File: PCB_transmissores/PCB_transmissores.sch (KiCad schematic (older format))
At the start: 17 parts, among them J2 Barrel_Jack_MountingPin

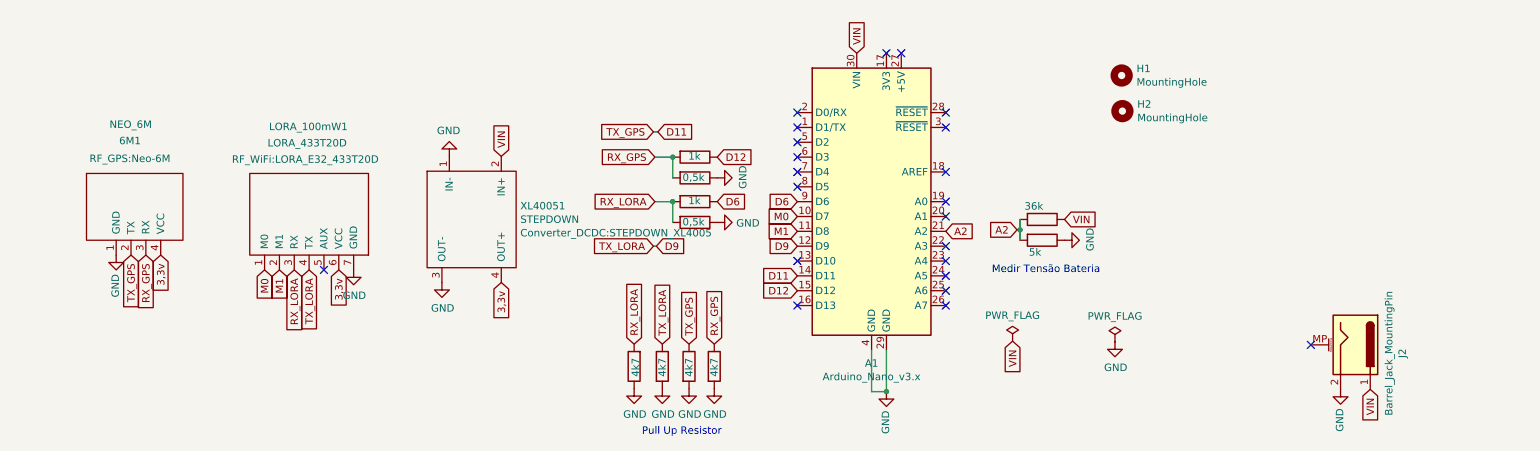
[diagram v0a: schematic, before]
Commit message: Atualização placa dos transmissores
Up
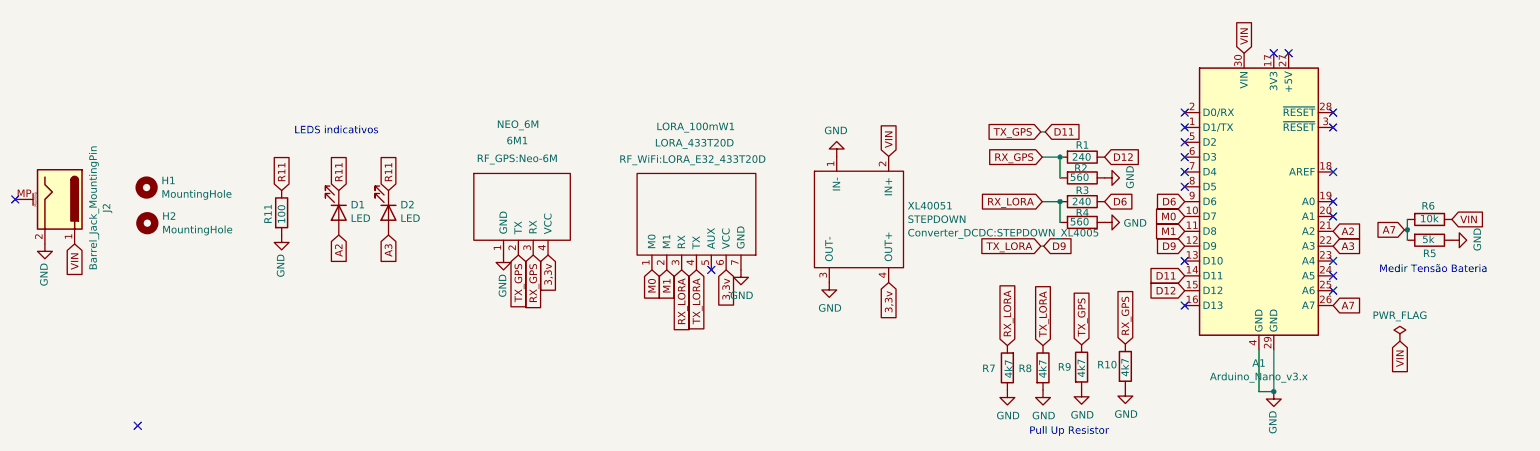
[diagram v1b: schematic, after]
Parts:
- added D1, D2: LED, LED_THT:LED_D5.0mm, symbol Device:LED
- added R11: 100, Resistor_THT:R_Axial_DIN0207_L6.3mm_D2.5mm_P7.62mm_Horizontal, symbol Device:R
- R1, R3: value 1k -> 240
- R2, R4: value 0,5k -> 560
- R6: value 36k -> 10k
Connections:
- net A2: now also D1.2 (A); no longer R5.2, R6.2
- net GND: now also R11.2
- net A3: now reaches A1.22 (A3)
- net A3: now also D2.2 (A)
- net A7: now reaches A1.26 (A7)
- net A7: now also R5.2, R6.2
- new net R11: D1.1 (K), D2.1 (K), R11.1
- no-connect marks 22 -> 21
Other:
- note added: "LEDS indicativos"
- moved on the sheet: 6M1, A1, H1, H2, J2, LORA_100mW1, XL40051
